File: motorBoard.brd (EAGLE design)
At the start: 69.5 x 80 mm, 20 parts, among them IC1 PIC18F4XK22PT

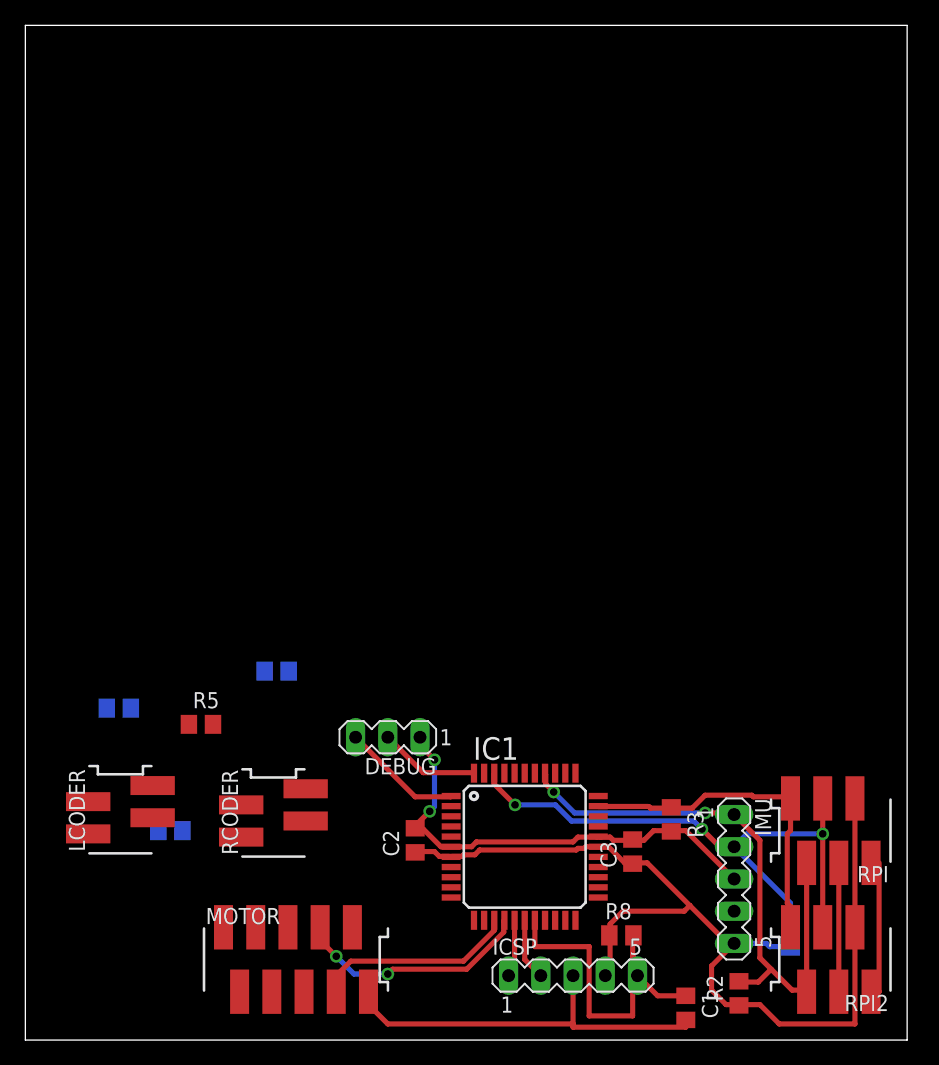
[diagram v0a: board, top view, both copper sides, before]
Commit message: board almost finished
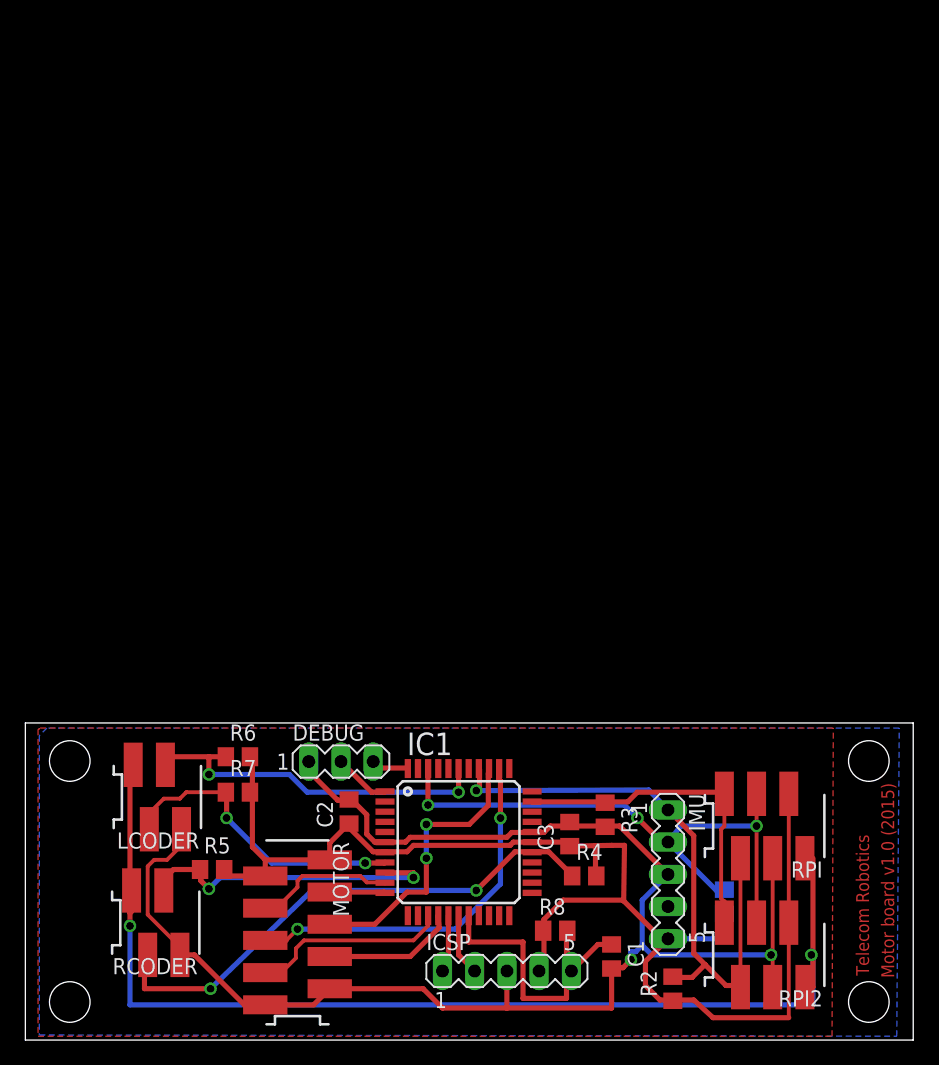
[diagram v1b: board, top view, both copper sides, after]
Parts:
- moved R4 29.1 mm to (44.1, 12.9), flipped to the top
- moved RCODER 12.7 mm to (10.3, 9.26), turned to 180 degrees
- moved R7 11.5 mm to (16.8, 19.5), flipped to the top
- moved R5 11.5 mm to (14.7, 13.4)
- moved R6 7.89 mm to (16.8, 22.3), flipped to the top, turned to 0 degrees
- moved C1 7.11 mm to (46.2, 6.59)
- moved R1 5.85 mm to (55.1, 10.9)
- moved C2 5.69 mm to (25.5, 18.0)
- moved IMU 5.23 mm to (50.7, 13.1)
- moved R2 5.23 mm to (51.0, 4.05)
- moved R8 5.23 mm to (41.8, 8.62)
- moved RPI 5.23 mm to (58.3, 16.9)
- moved RPI2 5.23 mm to (58.3, 6.71)
- moved IC1 5.23 mm to (34.2, 15.6)
- moved ICSP 5.23 mm to (38.0, 5.45)
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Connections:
- net N$12: now also DEBUG.2; no longer DEBUG.3
- net N$16: now also DEBUG.3; no longer DEBUG.2
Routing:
- net VDD: track 10.8 -> 87.9 mm, vias 0 -> 2
- net GND: track 78.0 -> 121.5 mm
- net N$1: track 0.00 -> 41.8 mm, vias 0 -> 2
- net VCC: track 79.5 -> 110.8 mm
- net N$4: track 0.00 -> 29.5 mm, vias 0 -> 2
- net N$11: track 0.00 -> 28.8 mm, vias 0 -> 2
- net N$13: track 0.00 -> 25.0 mm, vias 0 -> 2
- net N$7: track 0.00 -> 24.0 mm, vias 0 -> 2
- net N$23: track 0.00 -> 22.5 mm, vias 0 -> 2
- net N$3: track 0.00 -> 11.0 mm
- net N$8: track 18.9 -> 10.5 mm, vias 2 -> 0
- net N$12: track 9.52 -> 4.50 mm
- net N$16: track 7.96 -> 2.95 mm
- net N$2: track 0.00 -> 4.39 mm
- net N$18: track 27.8 -> 25.3 mm
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- added copper zone on layer 1, net N$10
- added copper zone on layer 16, net N$9
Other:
- board size 69.5 x 80 mm -> 70 x 25 mm
- board text added: "Motor board v1.0 (2015)"
- board text added: "Telecom Robotics"
